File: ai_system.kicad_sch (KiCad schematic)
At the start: 23 parts, among them U6 STM32N647L0H3Q

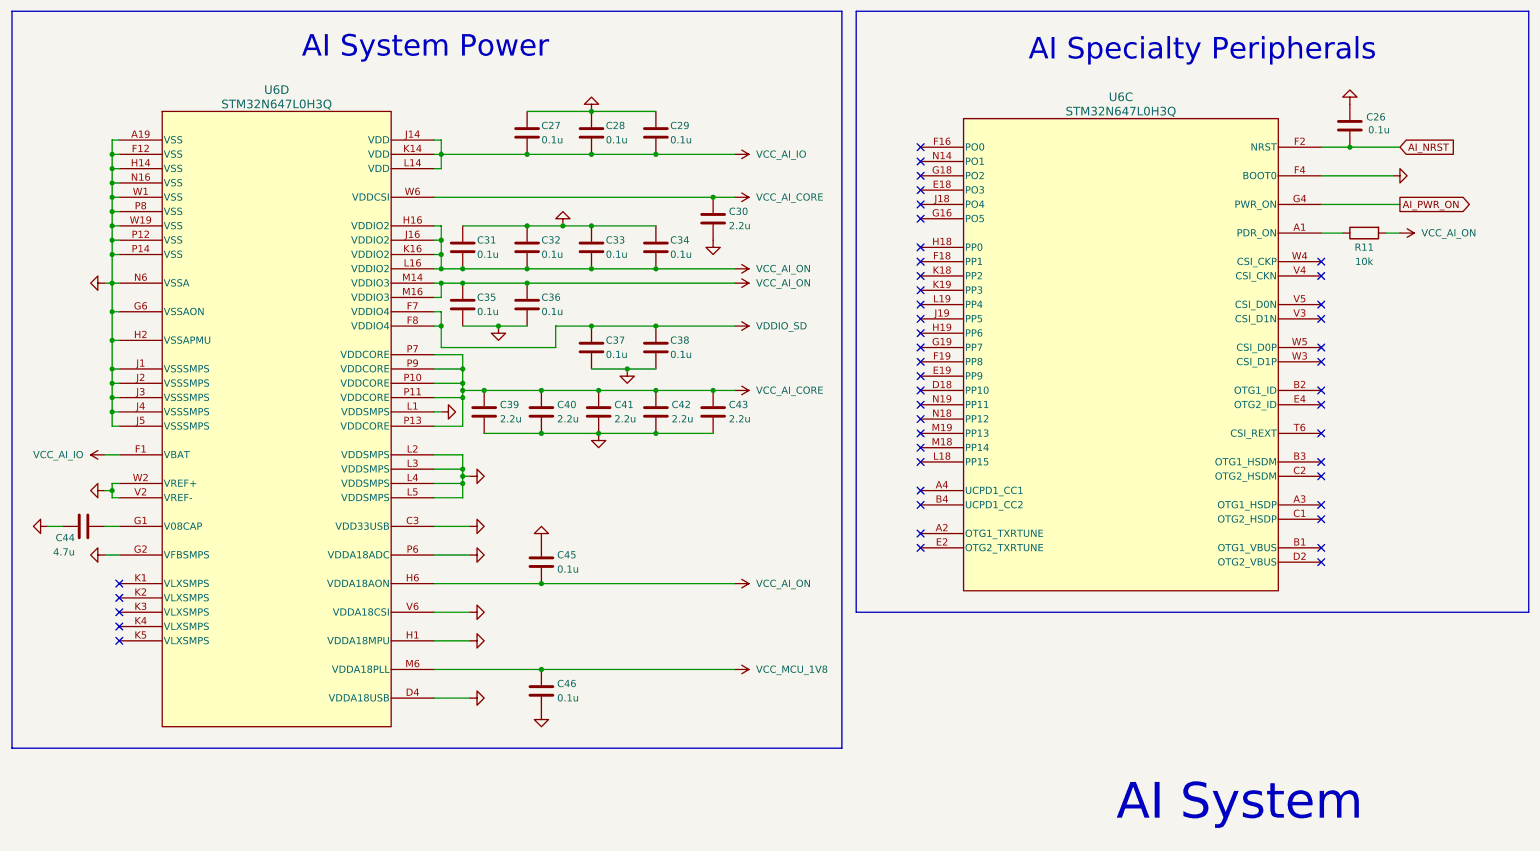
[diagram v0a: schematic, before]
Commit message: Updates for Rev. C
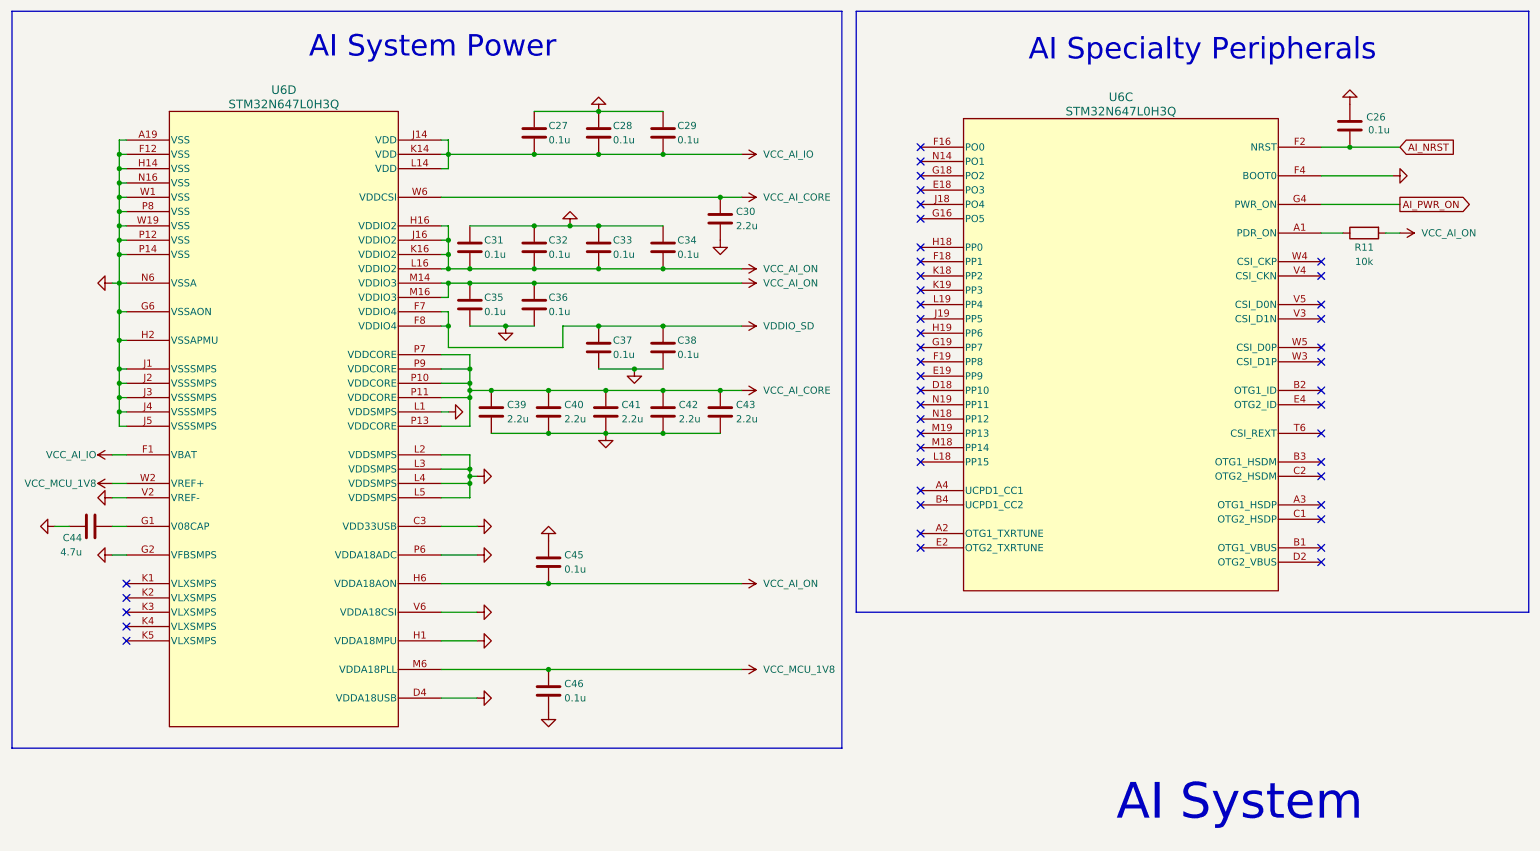
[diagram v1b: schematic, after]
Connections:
- net GND: no longer U6.W2 (VREF+)
- net VCC_MCU_1V8: now also U6.W2 (VREF+)
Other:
- moved on the sheet: C27, C28, C29, C30, C31, C32, C33, C34, C35, C36, C37, C38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
